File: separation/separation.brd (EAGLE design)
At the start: 9 parts, among them IC1 L7805ACV

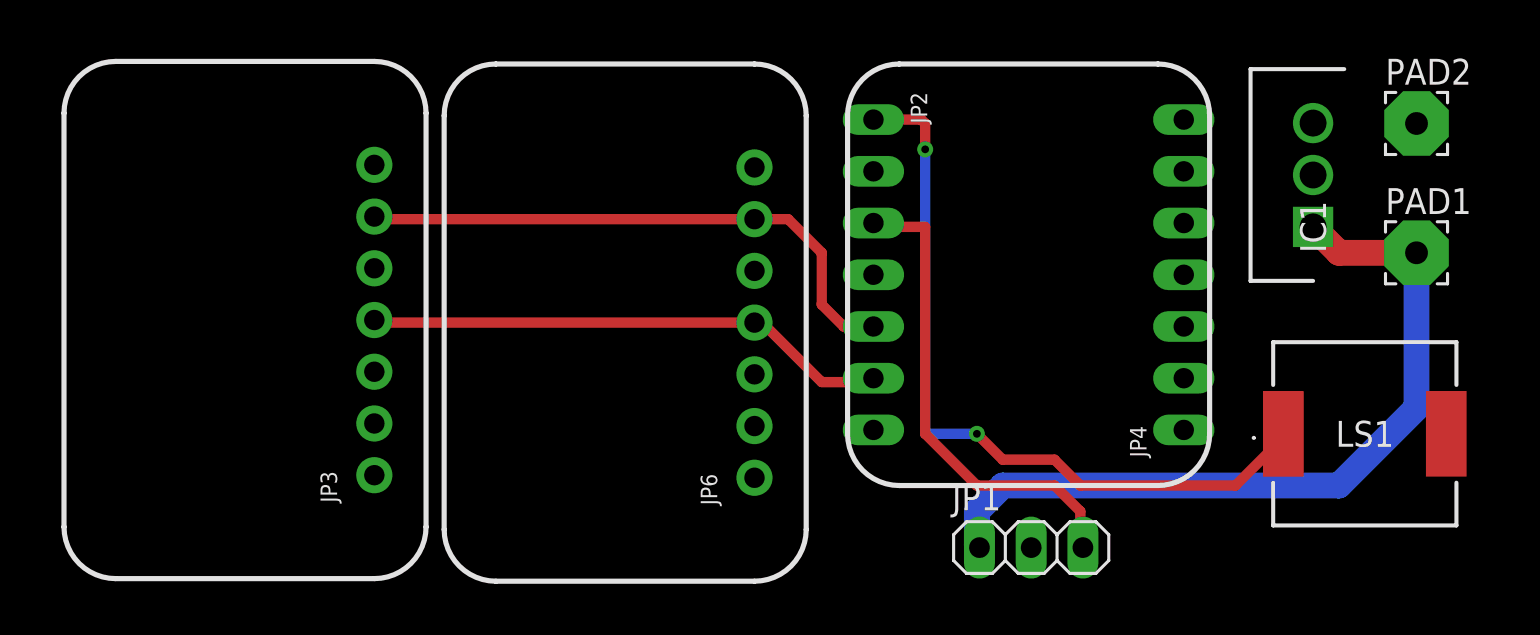
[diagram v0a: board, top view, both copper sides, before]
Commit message: create dimension
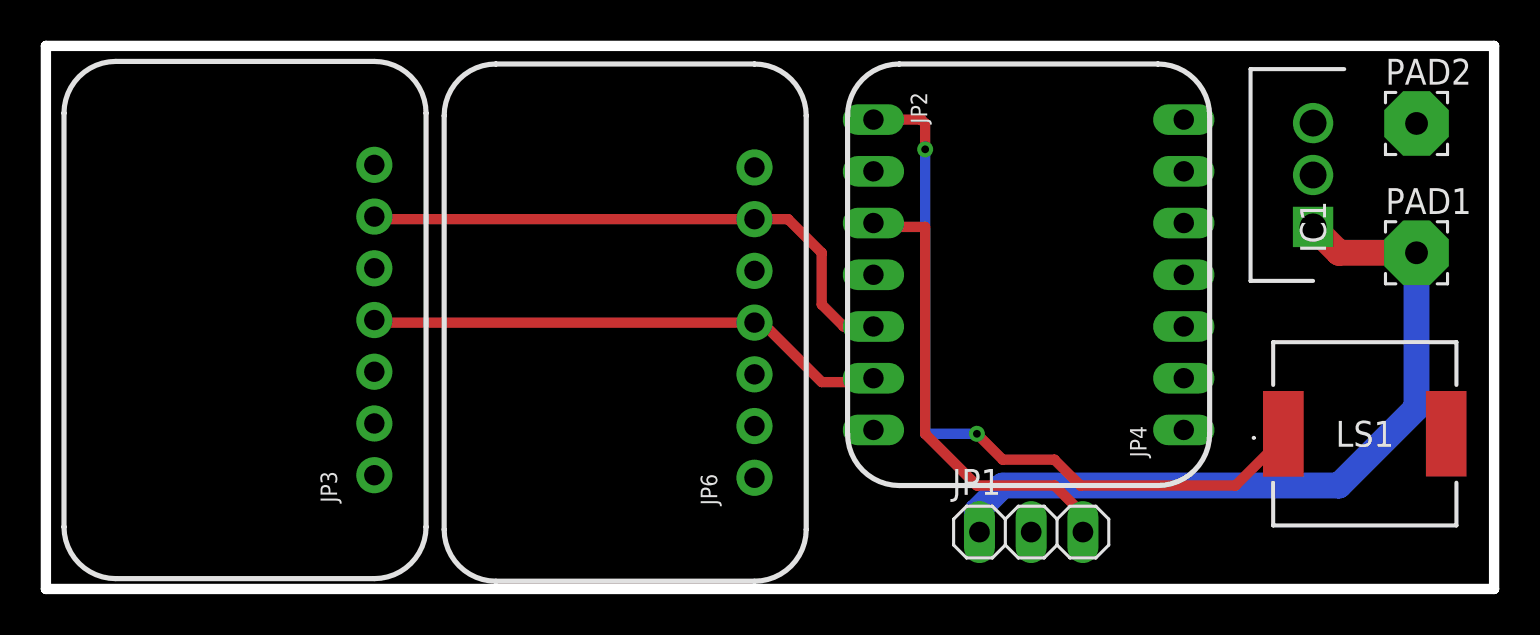
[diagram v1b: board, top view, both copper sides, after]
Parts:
- moved JP1 0.76 mm to (127.1, 54.9)
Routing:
- net VBAT: track 38.8 -> 38.0 mm
- net SERVO: track 23.8 -> 23.0 mm
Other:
- board outline added: 71.1 x 26.7 mm
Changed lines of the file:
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@@
 <wire x1="98.298" y1="75.311" x2="98.298" y2="54.991" width="0.254" layer="21"/>
 <wire x1="98.298" y1="54.991" x2="100.838" y2="52.451" width="0.254" layer="21" curve="90"/>
+<wire x1="78.74" y1="78.74" x2="149.86" y2="78.74" width="0.508" layer="20"/>
+<wire x1="149.86" y1="78.74" x2="149.86" y2="52.07" width="0.508" layer="20"/>
+<wire x1="149.86" y1="52.07" x2="78.74" y2="52.07" width="0.508" layer="20"/>
+<wire x1="78.74" y1="52.07" x2="78.74" y2="78.74" width="0.508" layer="20"/>
 </plain>
 <attributes>
@@
 <attribute name="VALUE" x="143.51" y="59.69" size="1.27" layer="27" align="center"/>
 </element>
-<element name="JP1" library="pinhead" library_urn="urn:adsk.eagle:library:325" package="1X03" package3d_urn="urn:adsk.eagle:package:22458/2" value="" x="127.127" y="54.102" smashed="yes">
-<attribute name="NAME" x="123.2408" y="55.9308" size="1.27" layer="25" ratio="10"/>
-<attribute name="POPULARITY" value="92" x="127.127" y="54.102" size="1.778" layer="27" font="vector" ratio="15" display="off"/>
-<attribute name="VALUE" x="123.317" y="50.927" size="1.27" layer="27"/>
+<element name="JP1" library="pinhead" library_urn="urn:adsk.eagle:library:325" package="1X03" package3d_urn="urn:adsk.eagle:package:22458/2" value="" x="127.127" y="54.864" smashed="yes">
+<attribute name="NAME" x="123.2408" y="56.6928" size="1.27" layer="25" ratio="10"/>
+<attribute name="POPULARITY" value="92" x="127.127" y="54.864" size="1.778" layer="27" font="vector" ratio="15" display="off"/>
+<attribute name="VALUE" x="123.317" y="51.689" size="1.27" layer="27"/>
 </element>
 <element name="PAD1" library="wirepad" library_urn="urn:adsk.eagle:library:412" package="3,17/1,1" package3d_urn="urn:adsk.eagle:package:30832/1" value="WIREPAD3,17/1,1" x="146.05" y="68.58" smashed="yes">
@@
 <wire x1="147.51" y1="59.69" x2="134.62" y2="72.5805" width="0" layer="19" extent="1-1"/>
 <wire x1="140.97" y1="72.4" x2="134.62" y2="72.5805" width="0" layer="19" extent="1-1"/>
-<wire x1="127.127" y1="54.102" x2="140.97" y2="72.4" width="0" layer="19" extent="1-1"/>
-<wire x1="146.05" y1="74.93" x2="127.127" y2="54.102" width="0" layer="19" extent="1-1"/>
+<wire x1="127.127" y1="54.864" x2="140.97" y2="72.4" width="0" layer="19" extent="1-1"/>
+<wire x1="146.05" y1="74.93" x2="127.127" y2="54.864" width="0" layer="19" extent="1-1"/>
 </signal>
 <signal name="A1">
@@
 <contactref element="JP1" pad="3"/>
 <wire x1="119.5705" y1="69.85" x2="119.38" y2="70.0405" width="0.508" layer="1"/>
-<wire x1="129.667" y1="54.102" x2="129.54" y2="54.229" width="0.508" layer="1"/>
-<wire x1="129.54" y1="54.229" x2="129.54" y2="55.88" width="0.508" layer="1"/>
+<wire x1="129.667" y1="54.864" x2="129.54" y2="54.991" width="0.508" layer="1"/>
+<wire x1="129.54" y1="54.991" x2="129.54" y2="55.88" width="0.508" layer="1"/>
 <wire x1="129.54" y1="55.88" x2="128.27" y2="57.15" width="0.508" layer="1"/>
 <wire x1="128.27" y1="57.15" x2="124.46" y2="57.15" width="0.508" layer="1"/>
@@
 <wire x1="146.05" y1="68.58" x2="142.24" y2="68.58" width="1.27" layer="1"/>
 <wire x1="142.24" y1="68.58" x2="140.97" y2="69.85" width="1.27" layer="1"/>
-<wire x1="124.587" y1="54.102" x2="124.46" y2="54.229" width="1.27" layer="16"/>
-<wire x1="124.46" y1="54.229" x2="124.46" y2="55.88" width="1.27" layer="16"/>
+<wire x1="124.587" y1="54.864" x2="124.46" y2="54.991" width="1.27" layer="16"/>
+<wire x1="124.46" y1="54.991" x2="124.46" y2="55.88" width="1.27" layer="16"/>
 <wire x1="124.46" y1="55.88" x2="125.73" y2="57.15" width="1.27" layer="16"/>
 <wire x1="125.73" y1="57.15" x2="142.24" y2="57.15" width="1.27" layer="16"/>
